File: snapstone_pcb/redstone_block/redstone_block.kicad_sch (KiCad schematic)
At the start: 4 parts, among them U2 XIAO-RP2040-NORMAL

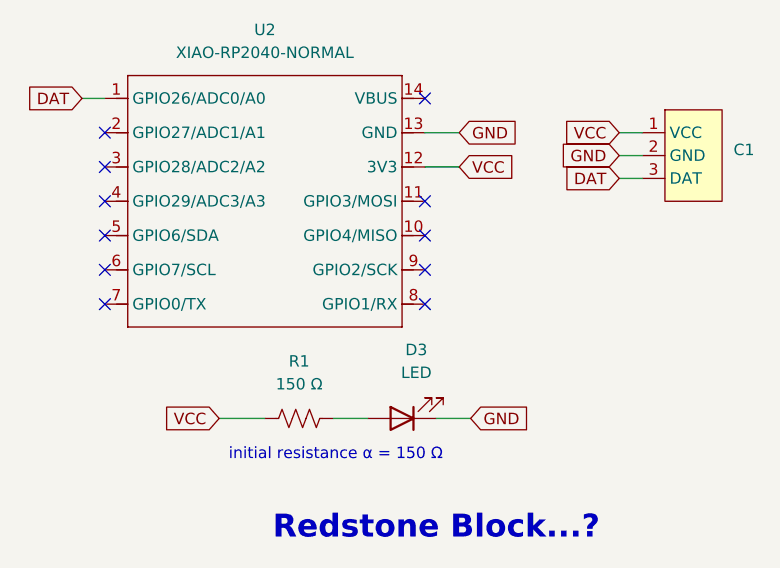
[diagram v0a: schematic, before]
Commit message: Added redstone comparator project!
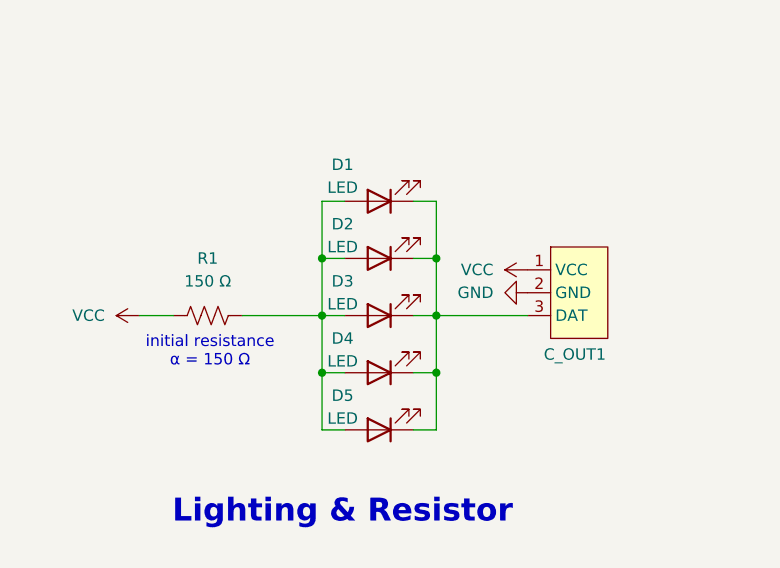
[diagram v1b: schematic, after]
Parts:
- removed U2: XIAO-RP2040-NORMAL, Module:MOUDLE14P-XIAO-DIP-SMD, symbol Seeed_Studio_XIAO_Series:XIAO-RP2040-NORMAL
- added D1, D2, D4, D5: LED, symbol Device:LED
- renumbered C1 to C_OUT1
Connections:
- net GND: no longer D3.1 (K)
- net at D3.2 (A), R1.1: now also D1.2 (A), D2.2 (A), D4.2 (A), D5.2 (A)
- net DAT: no longer names the net of C_OUT1.3 (DAT)
- net DAT: now also D3.1 (K), D1.1 (K), D2.1 (K), D4.1 (K), D5.1 (K)
- no-connect marks 11 -> 0
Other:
- note added: "Lighting & Resistor"
- note removed: "Redstone Block...?"
- moved on the sheet: C_OUT1, R1
